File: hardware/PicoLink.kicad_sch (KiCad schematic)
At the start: 51 parts, among them J2 USB_C_Receptacle_USB2.0_14P, J3 ARM_JTAG_10Pin, J4 TARGET, J7 UART, J8 SIGROK_INPUT, J9 SIGROK_ADC, SW2 BOOT SELECTOR, U2 74LVCH2T45DC, U4 W25Q16JVSS, U6 AMS1117-3.3, Y2 12Mhz HC49-SD

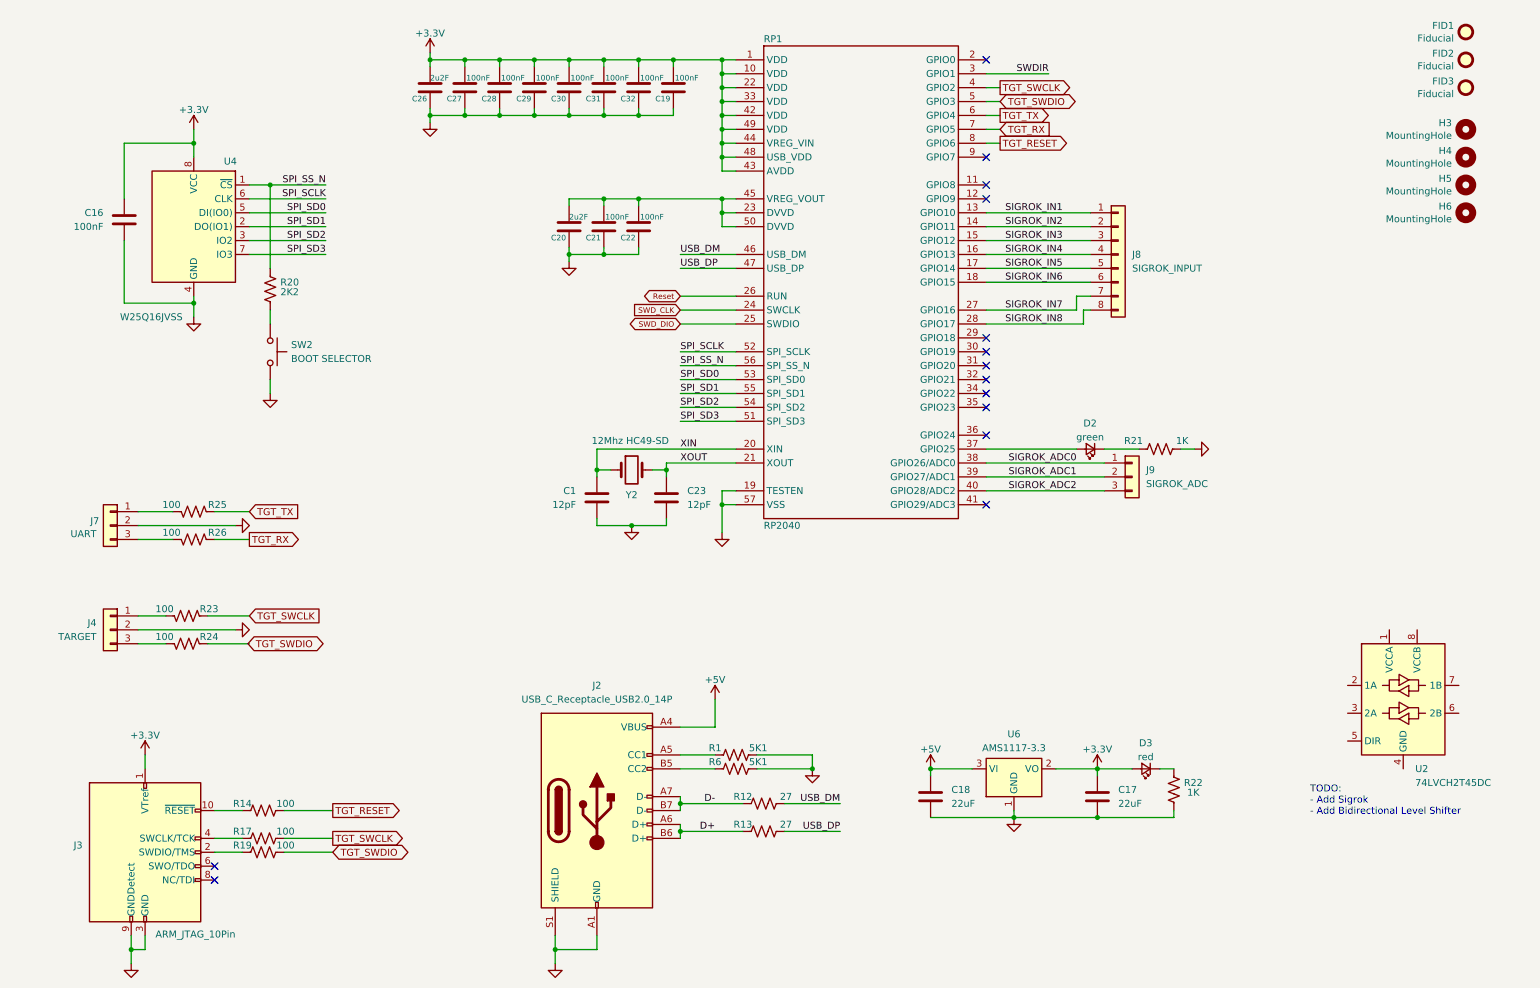
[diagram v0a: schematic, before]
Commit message: [07-20-0908] update gerber and schematic
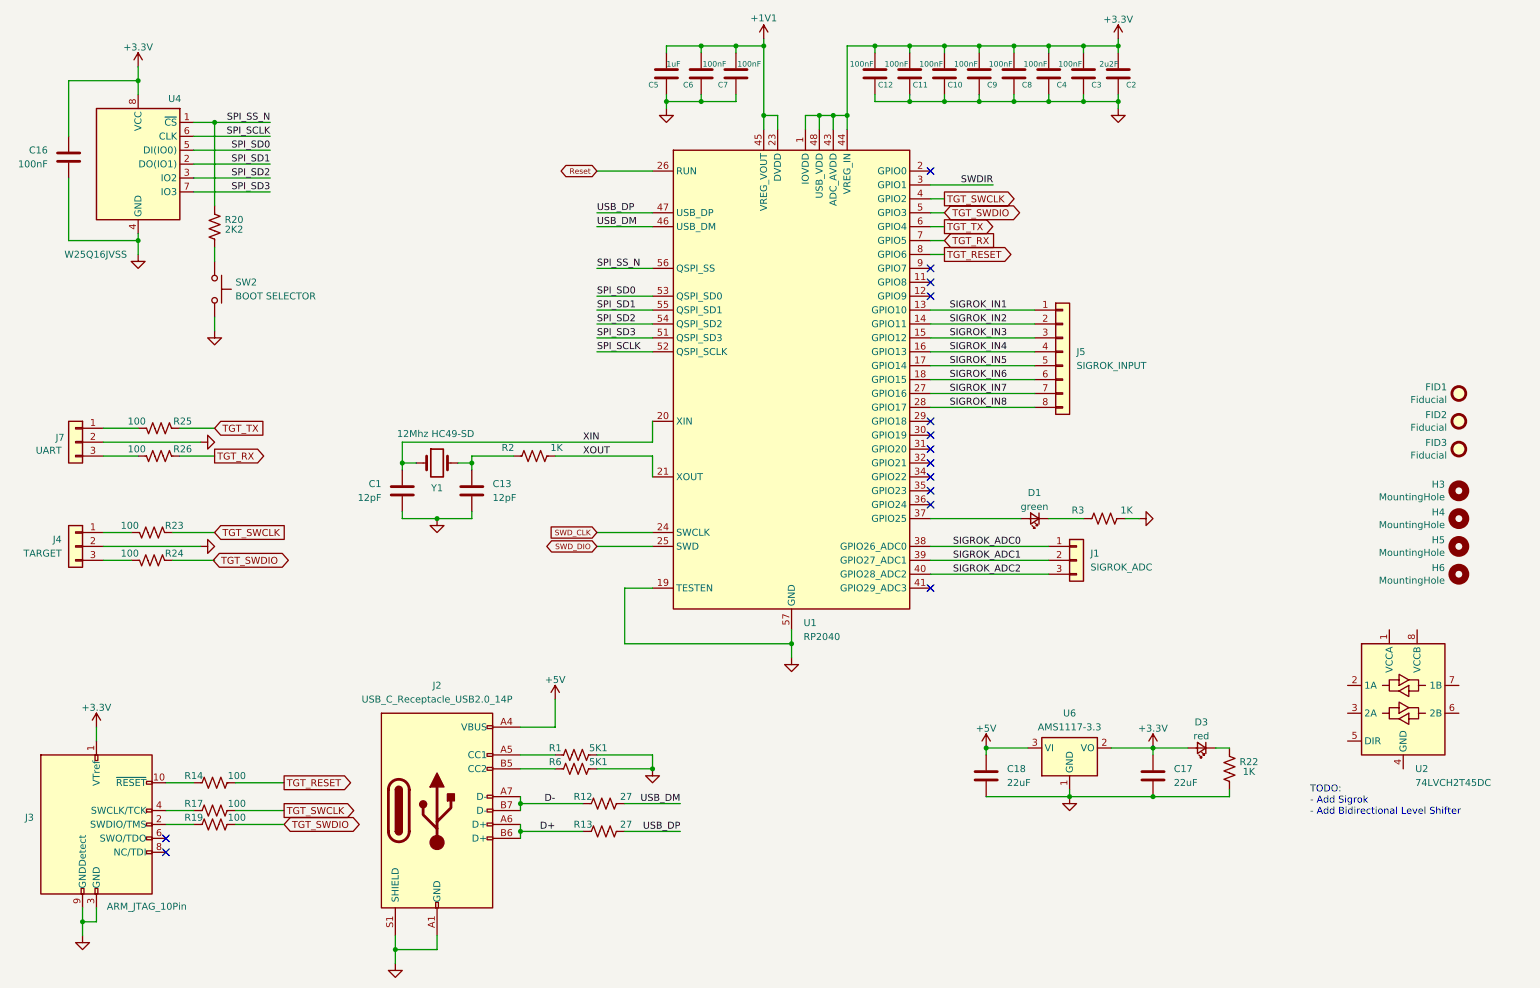
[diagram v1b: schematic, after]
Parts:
- removed C19, C21, C22, C27, C28, C29, C30, C31, C32: 100nF, Capacitor_SMD:C_0603_1608Metric_Pad1.08x0.95mm_HandSolder, symbol Device:C
- removed C20, C26: 2u2F, Capacitor_SMD:C_0603_1608Metric_Pad1.08x0.95mm_HandSolder, symbol Device:C
- removed C23: 12pF, Capacitor_SMD:C_0603_1608Metric_Pad1.08x0.95mm_HandSolder, symbol Device:C
- removed D2: green, LED_SMD:LED_0805_2012Metric_Pad1.15x1.40mm_HandSolder, symbol Device:LED_Small
- removed J8: SIGROK_INPUT, Connector_PinHeader_2.54mm:PinHeader_1x07_P2.54mm_Vertical, symbol Connector_Generic:Conn_01x08
- removed J9: SIGROK_ADC, Connector_PinHeader_2.54mm:PinHeader_1x03_P2.54mm_Vertical, symbol Connector_Generic:Conn_01x03
- removed R21: 1K, Resistor_SMD:R_0805_2012Metric_Pad1.20x1.40mm_HandSolder, symbol Device:R_US
- removed RP1: RP2040, Package_DFN_QFN:QFN-56-1EP_7x7mm_P0.4mm_EP3.2x3.2mm, symbol McuOnEclipse:RP2040
- removed Y2: 12Mhz HC49-SD, Crystal:Crystal_SMD_HC49-SD_HandSoldering, symbol Device:Crystal
- added C10, C11, C12, C3, C4, C6, C7, C8, C9: 100nF, Capacitor_SMD:C_0603_1608Metric_Pad1.08x0.95mm_HandSolder, symbol Device:C
- added C13: 12pF, Capacitor_SMD:C_0603_1608Metric_Pad1.08x0.95mm_HandSolder, symbol Device:C
- added C2: 2u2F, Capacitor_SMD:C_0603_1608Metric_Pad1.08x0.95mm_HandSolder, symbol Device:C
- added C5: 1uF, Capacitor_SMD:C_0603_1608Metric_Pad1.08x0.95mm_HandSolder, symbol Device:C
- added D1: green, LED_SMD:LED_0805_2012Metric_Pad1.15x1.40mm_HandSolder, symbol Device:LED_Small
- added J1: SIGROK_ADC, Connector_PinHeader_2.54mm:PinHeader_1x03_P2.54mm_Vertical, symbol Connector_Generic:Conn_01x03
- added J5: SIGROK_INPUT, Connector_PinHeader_2.54mm:PinHeader_1x07_P2.54mm_Vertical, symbol Connector_Generic:Conn_01x08
- added R2, R3: 1K, Resistor_SMD:R_0805_2012Metric_Pad1.20x1.40mm_HandSolder, symbol Device:R_US
- added U1: RP2040, Package_DFN_QFN:QFN-56-1EP_7x7mm_P0.4mm_EP3.2x3.2mm, symbol MCU_RaspberryPi:RP2040
- added Y1: 12Mhz HC49-SD, Crystal:Crystal_SMD_HC49-SD, symbol Device:Crystal
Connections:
- net +3.3V: now also C10.1, C11.1, C12.1, C2.1, C3.1, C4.1, C8.1, C9.1, U1.1 (IOVDD), U1.10 (IOVDD), U1.22 (IOVDD), U1.33 (IOVDD), U1.42 (IOVDD), U1.43 (ADC_AVDD), U1.44 (VREG_IN), U1.48 (USB_VDD), U1.49 (IOVDD)
- net GND: now also C10.2, C11.2, C12.2, C13.2, C2.2, C3.2, C4.2, C5.2, C6.2, C7.2, C8.2, C9.2, R3.2, U1.19 (TESTEN), U1.57 (GND)
- net Reset: now also U1.26 (RUN)
- net SIGROK_ADC0: now also J1.1 (Pin_1), U1.38 (GPIO26_ADC0)
- net SIGROK_ADC1: now also J1.2 (Pin_2), U1.39 (GPIO27_ADC1)
- net SIGROK_ADC2: now also J1.3 (Pin_3), U1.40 (GPIO28_ADC2)
- net SIGROK_IN1: now also J5.1 (Pin_1), U1.13 (GPIO10)
- net SIGROK_IN2: now also J5.2 (Pin_2), U1.14 (GPIO11)
- net SIGROK_IN3: now also J5.3 (Pin_3), U1.15 (GPIO12)
- net SIGROK_IN4: now also J5.4 (Pin_4), U1.16 (GPIO13)
- net SIGROK_IN5: now also J5.5 (Pin_5), U1.17 (GPIO14)
- net SIGROK_IN6: now also J5.6 (Pin_6), U1.18 (GPIO15)
- net SIGROK_IN7: now also J5.7 (Pin_7), U1.27 (GPIO16)
- net SIGROK_IN8: now also J5.8 (Pin_8), U1.28 (GPIO17)
- net SPI_SCLK: now also U1.52 (QSPI_SCLK)
- net SPI_SD0: now also U1.53 (QSPI_SD0)
- net SPI_SD1: now also U1.55 (QSPI_SD1)
- net SPI_SD2: now also U1.54 (QSPI_SD2)
- net SPI_SD3: now also U1.51 (QSPI_SD3)
- net SPI_SS_N: now also U1.56 (QSPI_SS)
- net SWDIR: now also U1.3 (GPIO1)
- net SWD_CLK: now also U1.24 (SWCLK)
- net SWD_DIO: now also U1.25 (SWD)
- net TGT_RESET: now also U1.8 (GPIO6)
- net TGT_RX: now also U1.7 (GPIO5)
- net TGT_SWCLK: now also U1.4 (GPIO2)
- net TGT_SWDIO: now also U1.5 (GPIO3)
- net TGT_TX: now also U1.6 (GPIO4)
- net USB_DM: now also U1.46 (USB_DM)
- net USB_DP: now also U1.47 (USB_DP)
- net XIN: now also U1.20 (XIN), Y1.1
- net XOUT: now also R2.2, U1.21 (XOUT)
- new net: D1.1 (K), R3.1
- new net: D1.2 (A), U1.37 (GPIO25)
- new net: C13.1, R2.1, Y1.2
- new net +1V1: C5.1, C6.1, C7.1, U1.23 (DVDD), U1.45 (VREG_VOUT), U1.50 (DVDD)
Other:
- moved on the sheet: C16, C17, C18, D3, FID1, FID2, FID3, H3, H4, H5, H6, J2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
